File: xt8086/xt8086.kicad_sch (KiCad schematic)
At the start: 21 parts, among them J1 UART, J12 8086_Pins_Right, J2 DEBUG, J3 8086_Pins_Left, U1 SN74LS04, U2 SN74LS74

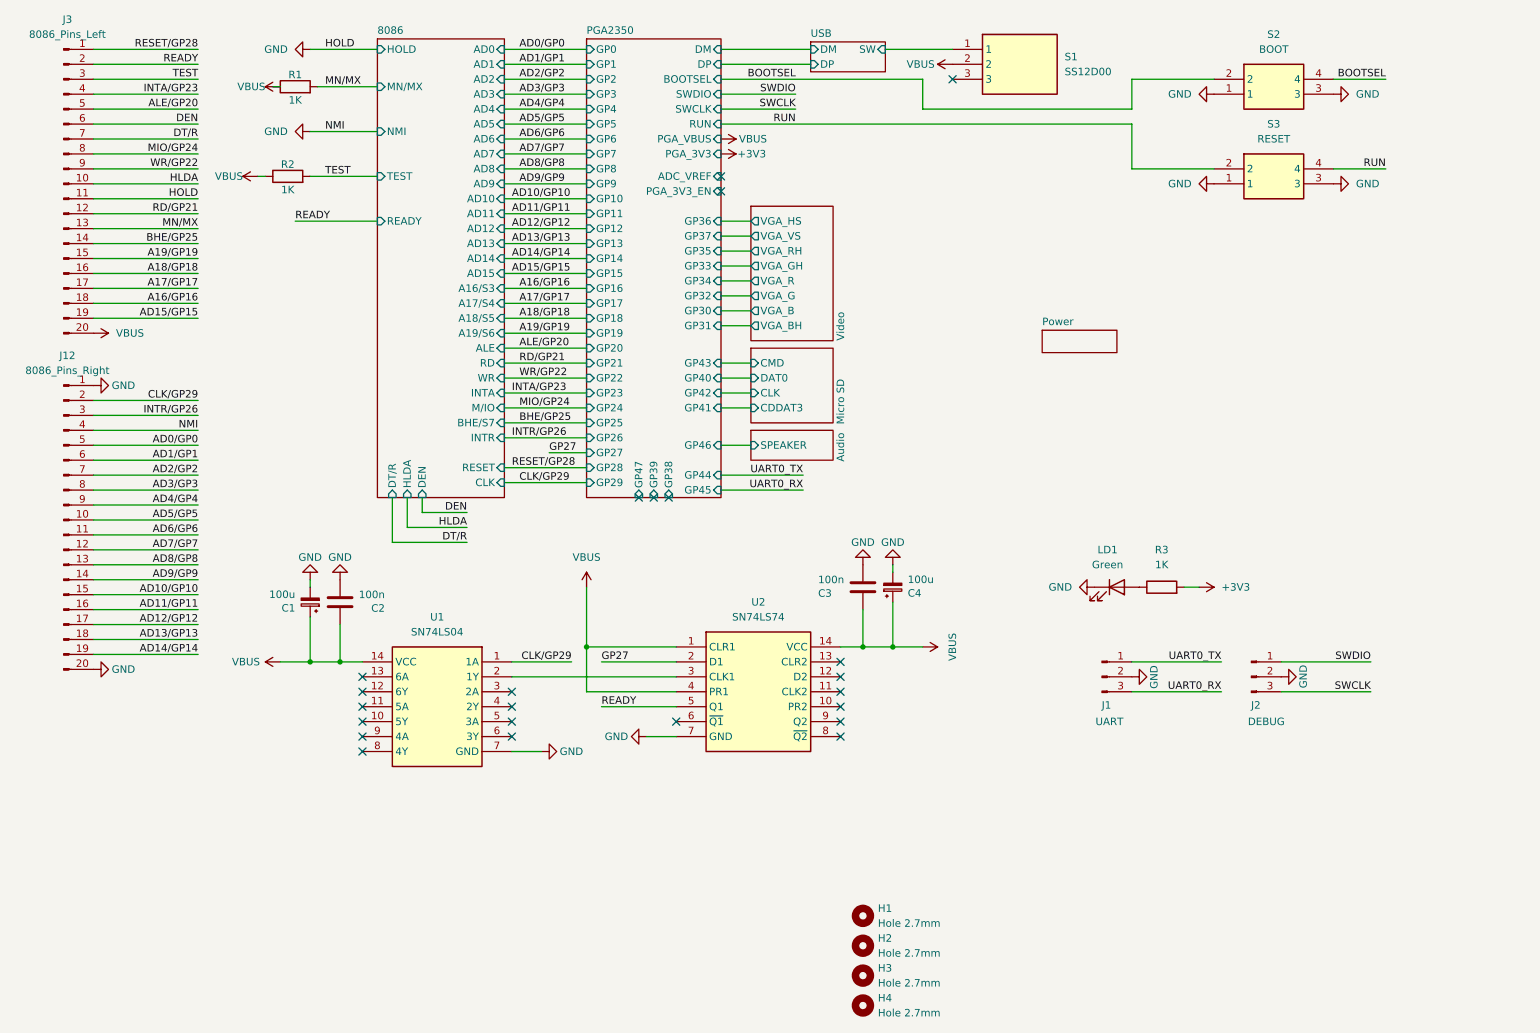
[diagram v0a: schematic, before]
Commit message: xt8086 1.03
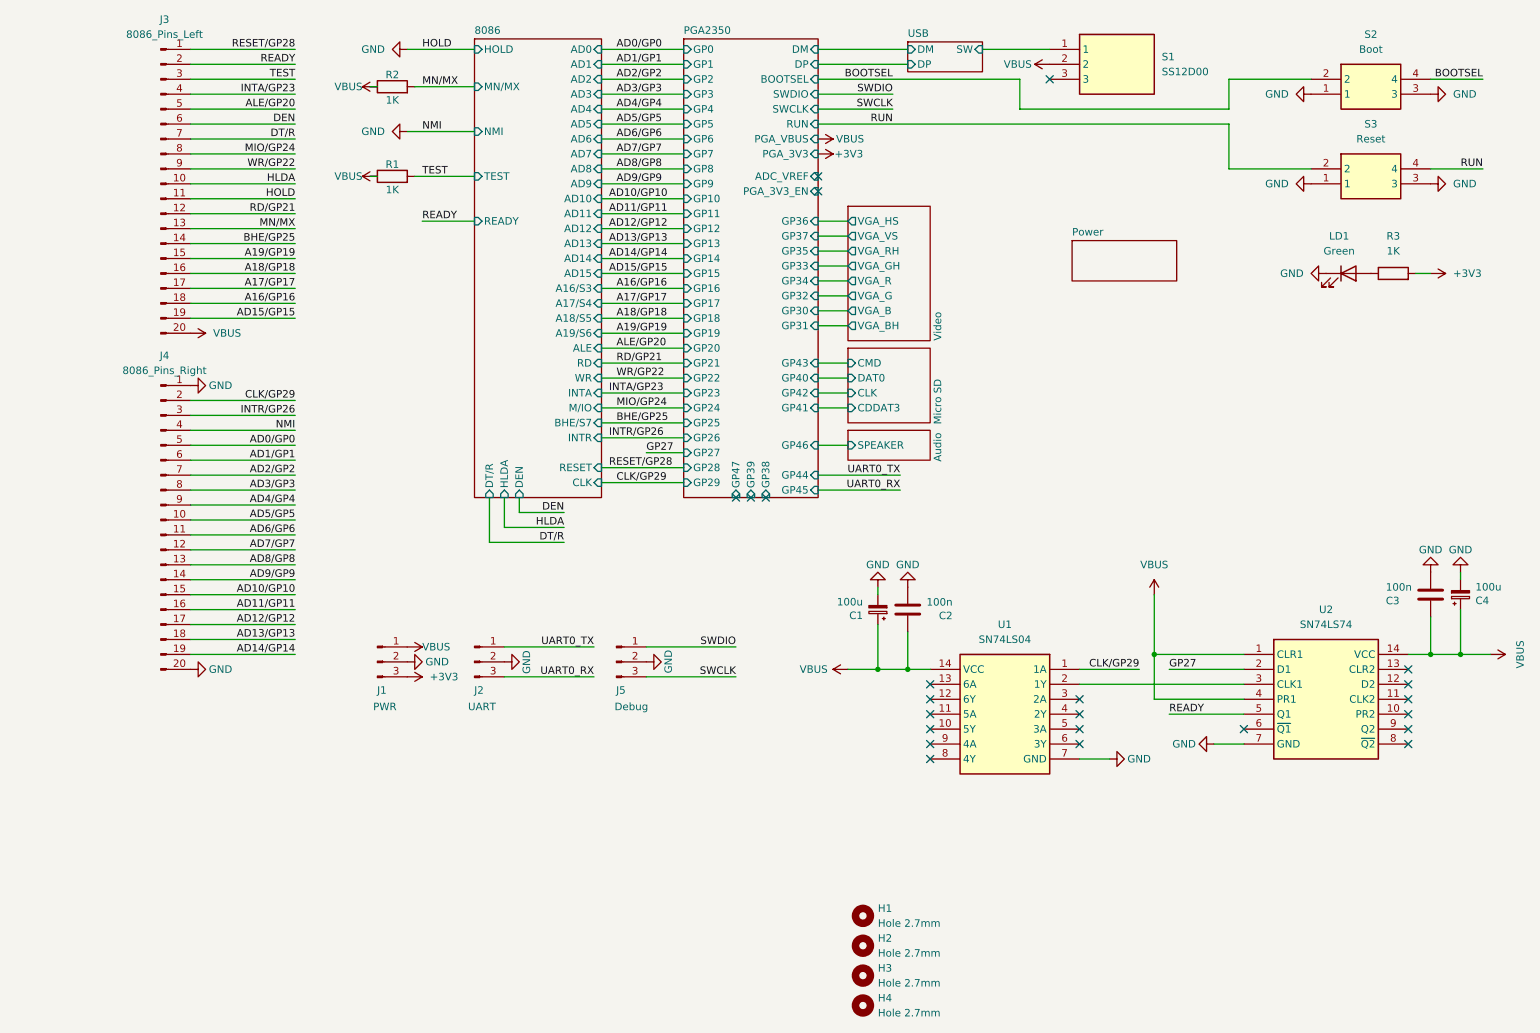
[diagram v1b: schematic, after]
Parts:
- added J1: PWR, xt8086:PinHeader_1x03_P2.54mm_Vertical, symbol xt8086:Conn_01x03_Pin
- J5: renamed from J2; value DEBUG -> Debug
- S2: value BOOT -> Boot
- S3: value RESET -> Reset
- renumbered J1 to J2, J12 to J4, R2 to R1, R1 to R2
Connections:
- net +3V3: now also J1.3 (Pin_3)
- net GND: now also J1.2 (Pin_2)
- net VBUS: now also J1.1 (Pin_1)
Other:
- moved on the sheet: C1, C2, C3, C4, J2, J3, J4, J5, LD1, R1, R2, R3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
